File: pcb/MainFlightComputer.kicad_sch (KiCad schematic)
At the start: 73 parts, among them J1 614105150721, J3 Micro_SD_Card, J4 Pinout, J5 Debug, SW1 B3U-1000P, SW2 B3U-1000P, U1 STM32H533VET6, U2 MCP2221A-I/ST, U3 AP2112K-3.3

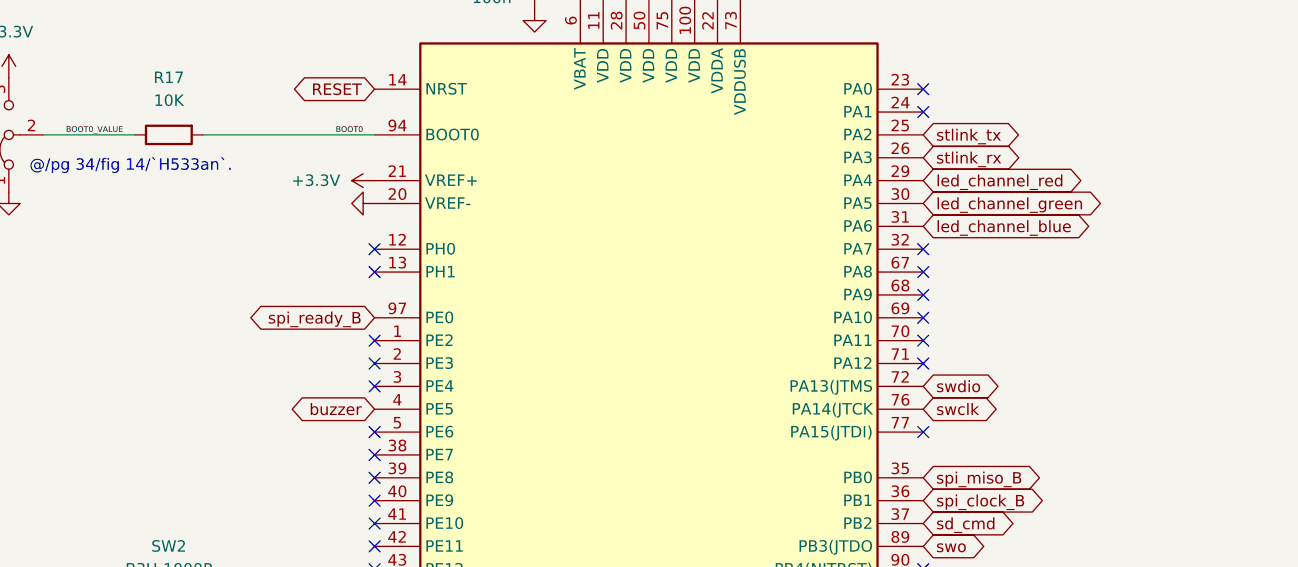
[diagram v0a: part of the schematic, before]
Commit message: Routed `led_channel_x`.
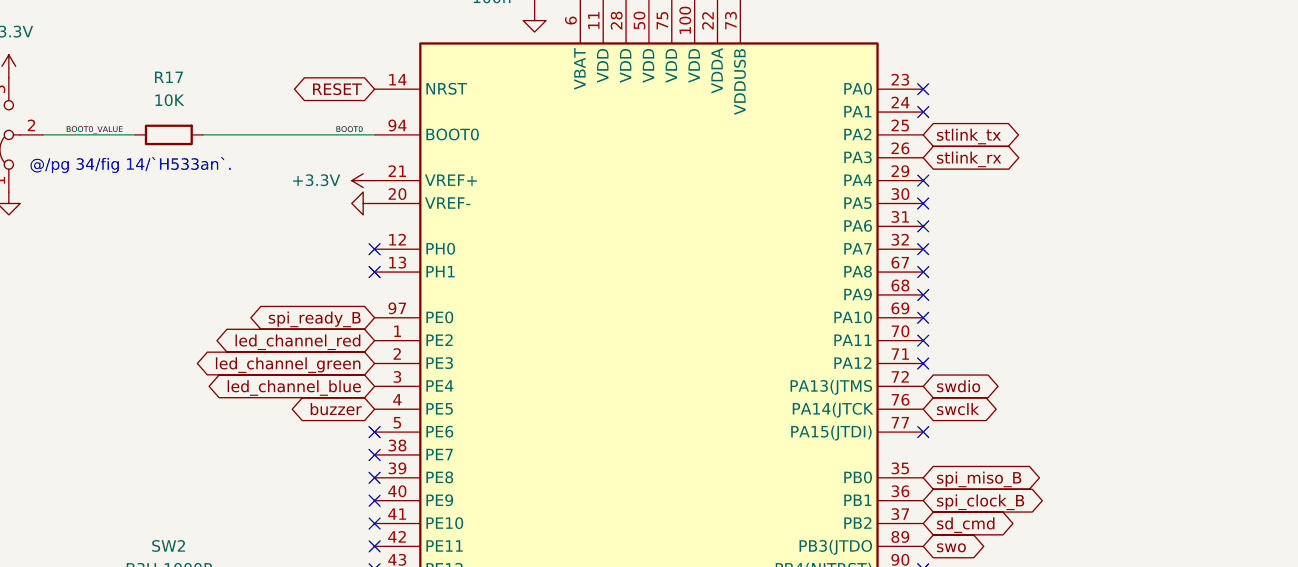
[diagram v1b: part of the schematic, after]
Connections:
- net led_channel_blue: now also U1.3 (PE4); no longer U1.31 (PA6)
- net led_channel_green: now also U1.2 (PE3); no longer U1.30 (PA5)
- net led_channel_red: now also U1.1 (PE2); no longer U1.29 (PA4)
